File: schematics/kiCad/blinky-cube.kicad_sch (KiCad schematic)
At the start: 11 parts, among them J1 Screw_Terminal_01x02, J2 Screw_Terminal_01x03, J3 Screw_Terminal_01x03, SW1 SW_Push, U1 Pico

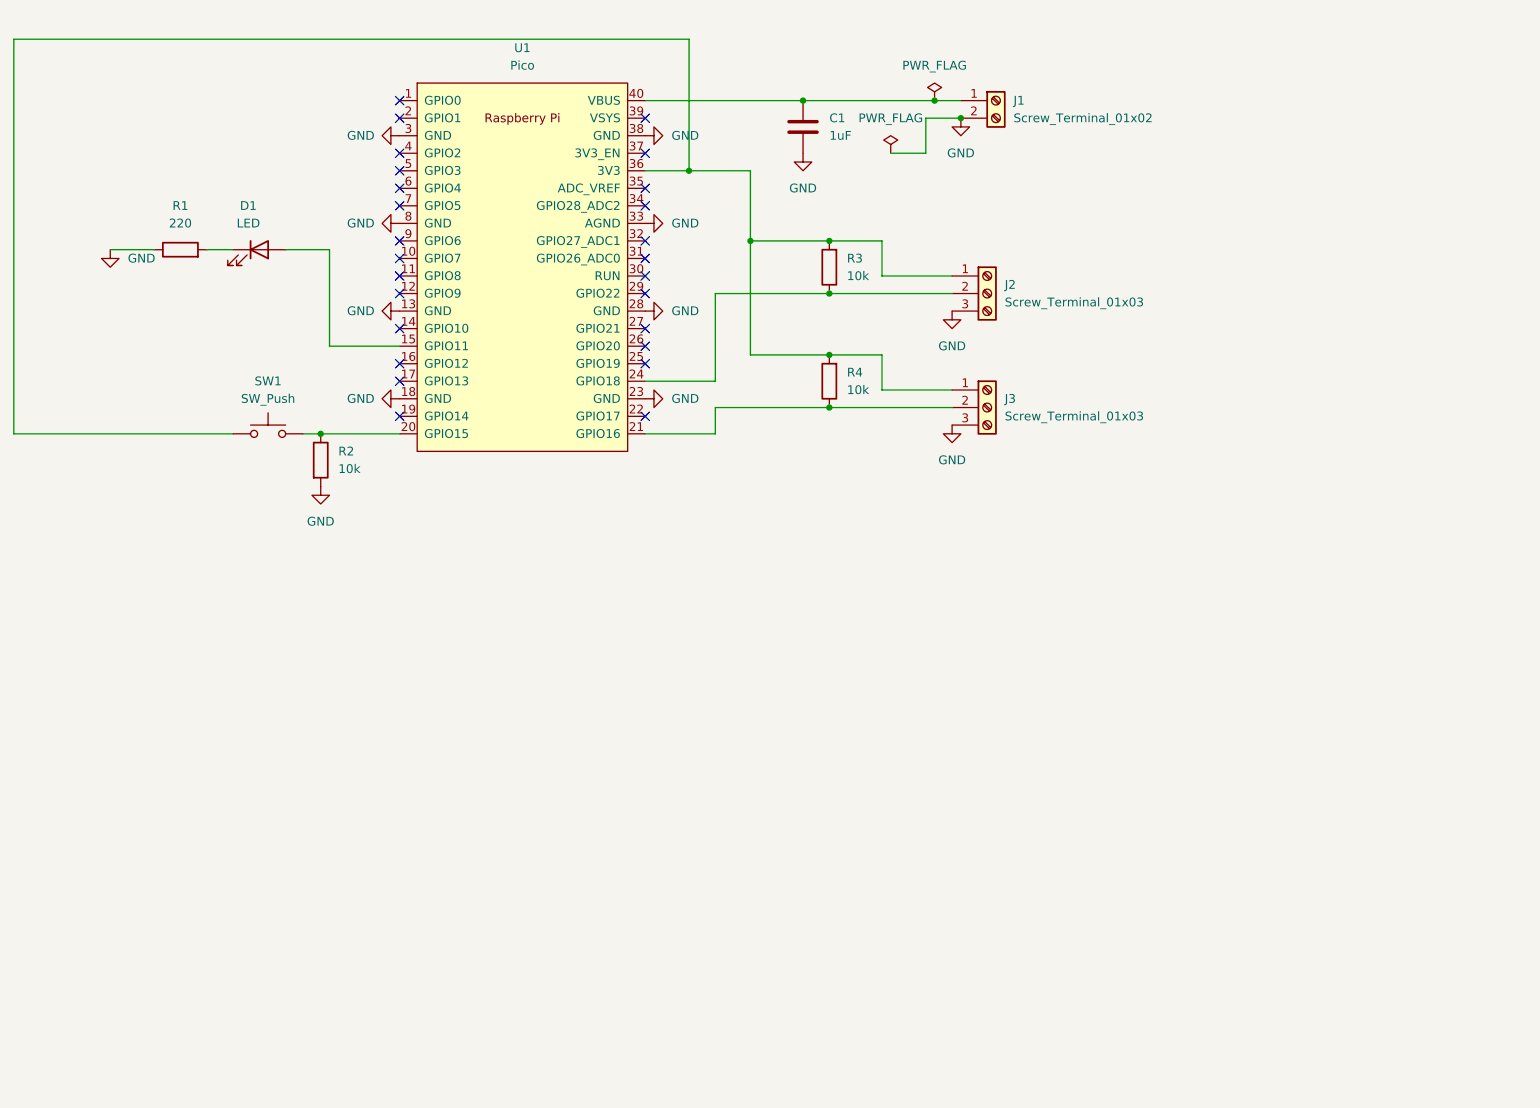
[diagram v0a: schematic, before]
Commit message: schematic in DIN mode 3 format
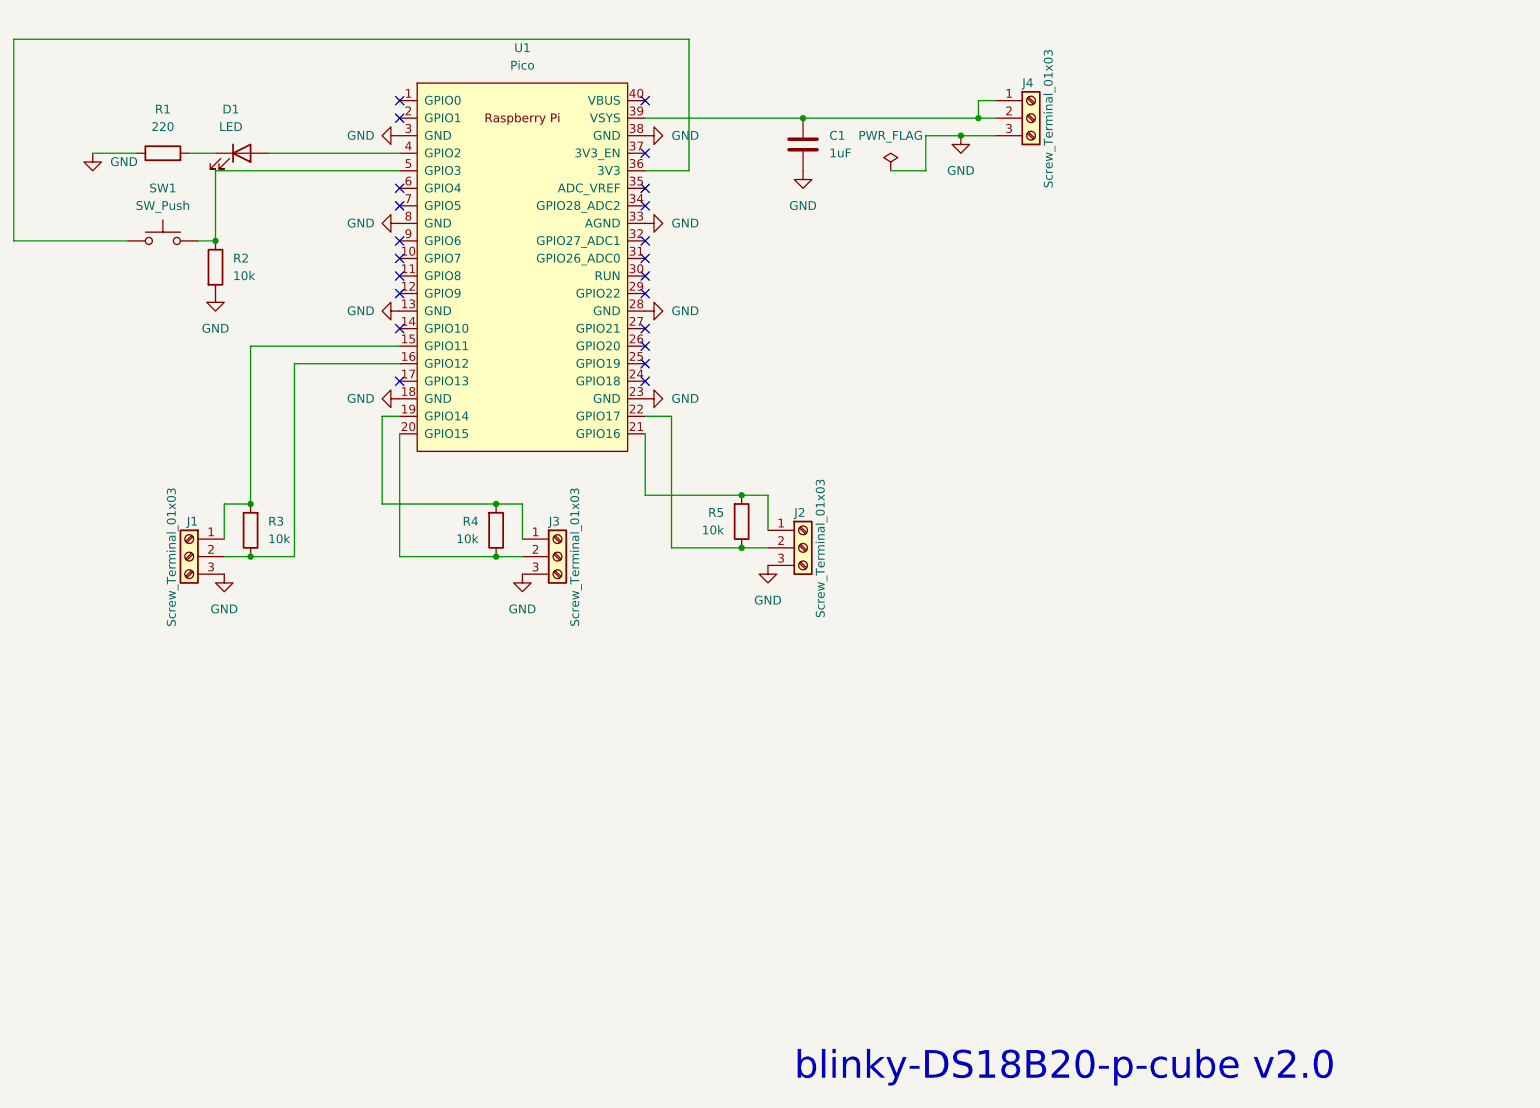
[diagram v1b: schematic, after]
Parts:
- removed J1: Screw_Terminal_01x02, TerminalBlock:TerminalBlock_bornier-2_P5.08mm, symbol Connector:Screw_Terminal_01x02
- added J1, J4: Screw_Terminal_01x03, TerminalBlock:TerminalBlock_bornier-3_P5.08mm, symbol Connector:Screw_Terminal_01x03
- added R5: 10k, Resistor_SMD:R_1206_3216Metric_Pad1.30x1.75mm_HandSolder, symbol Device:R
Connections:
- net GND: now also J1.3 (Pin_3), J4.3 (Pin_3)
- net at R2.1, SW1.2: now also U1.5 (GPIO3); no longer U1.20 (GPIO15)
- net at C1.1: now also U1.39 (VSYS), J4.1 (Pin_1), J4.2 (Pin_2); no longer U1.40 (VBUS)
- net at U1.15 (GPIO11): now also R3.2, J1.1 (Pin_1); no longer D1.2 (A)
- net at U1.16 (GPIO12): now also R3.1, J1.2 (Pin_2)
- net at U1.19 (GPIO14): now also J3.1 (Pin_1), R4.2
- net at J3.2 (Pin_2), R4.1: now also U1.20 (GPIO15); no longer U1.21 (GPIO16)
- net at U1.22 (GPIO17): now also J2.2 (Pin_2), R5.1
- net at U1.4 (GPIO2): now also D1.2 (A)
- new net: J2.1 (Pin_1), R5.2, U1.21 (GPIO16)
- new net: SW1.1, U1.36 (3V3)
- now unconnected: U1.24 (GPIO18)
- no-connect marks 26 -> 22
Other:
- note added: "blinky-DS18B20-p-cube v2.0"
- moved on the sheet: C1, D1, R1, R2, SW1
